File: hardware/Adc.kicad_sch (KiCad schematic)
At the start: 36 parts

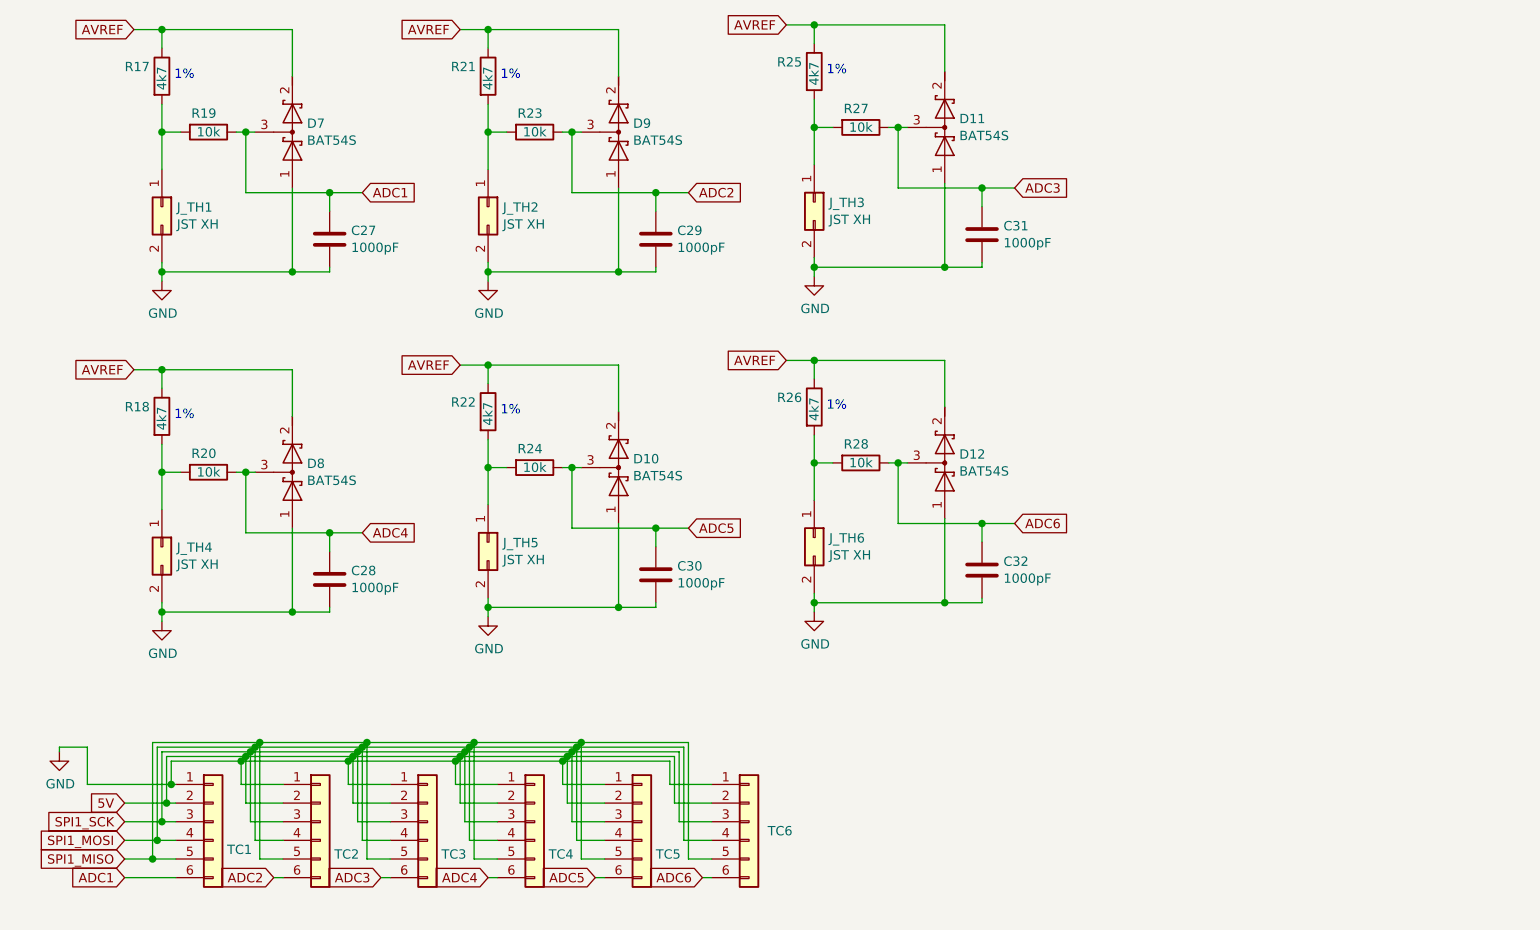
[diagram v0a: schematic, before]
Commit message: Intermediate checkin
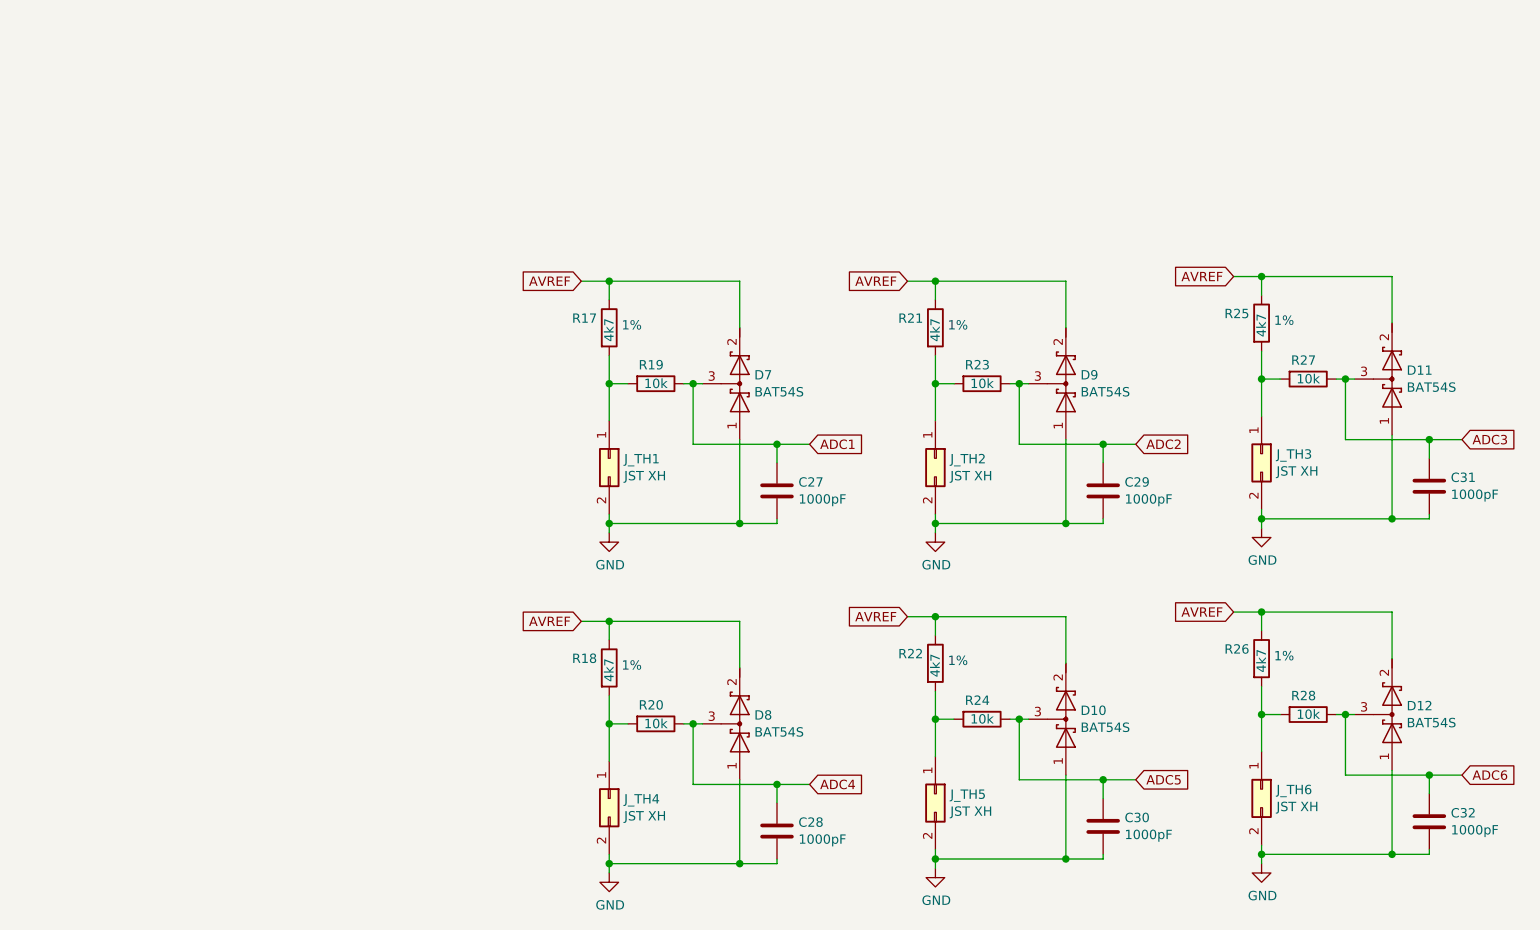
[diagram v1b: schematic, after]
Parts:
- removed TC1, TC2, TC3, TC4, TC5, TC6: TC, kicad-molex-sl-footprints:Molex-SL-6POS, symbol Connector_Generic:Conn_01x06
- C27, C28, C29, C30, C31, C32: footprint PrntrBoardV2:C_0603_1608Metric -> Capacitor_SMD:C_0402_1005Metric; LCSC Part # C1588 -> C1523; Part # CL10B102KB8NNNC -> 0402B102K500NT
- R17, R18, R21, R22, R25, R26: footprint PrntrBoardV2:R_0603_1608Metric -> Resistor_SMD:R_0402_1005Metric; LCSC Part # C23162 -> C25900; Part # 0603WAF4701T5E -> 0402WGF4701TCE
- R19, R20, R23, R24, R27, R28: footprint PrntrBoardV2:R_0603_1608Metric -> Resistor_SMD:R_0402_1005Metric; LCSC Part # C25804 -> C25744; Part # 0603WAF1002T5E -> 0402WGF1002TCE
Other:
- moved on the sheet: C27, C28, C29, C30, C31, C32, D10, D11, D12, D7, D8, D9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
